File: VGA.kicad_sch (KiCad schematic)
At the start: 15 parts, among them U5 LMH6881SQ/NOPB

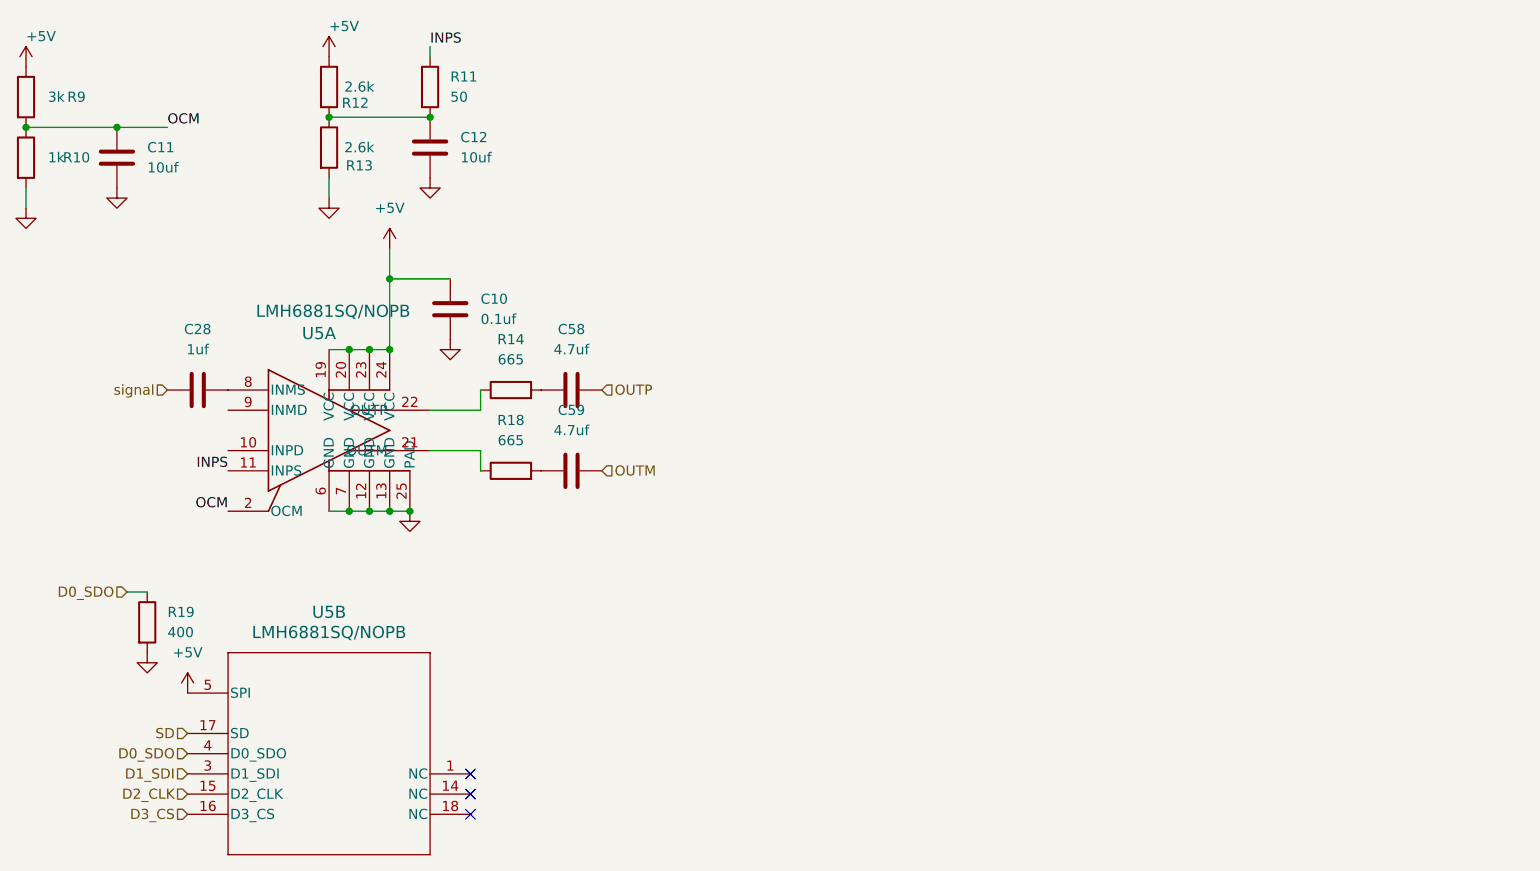
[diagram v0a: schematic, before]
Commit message: routing draft 2
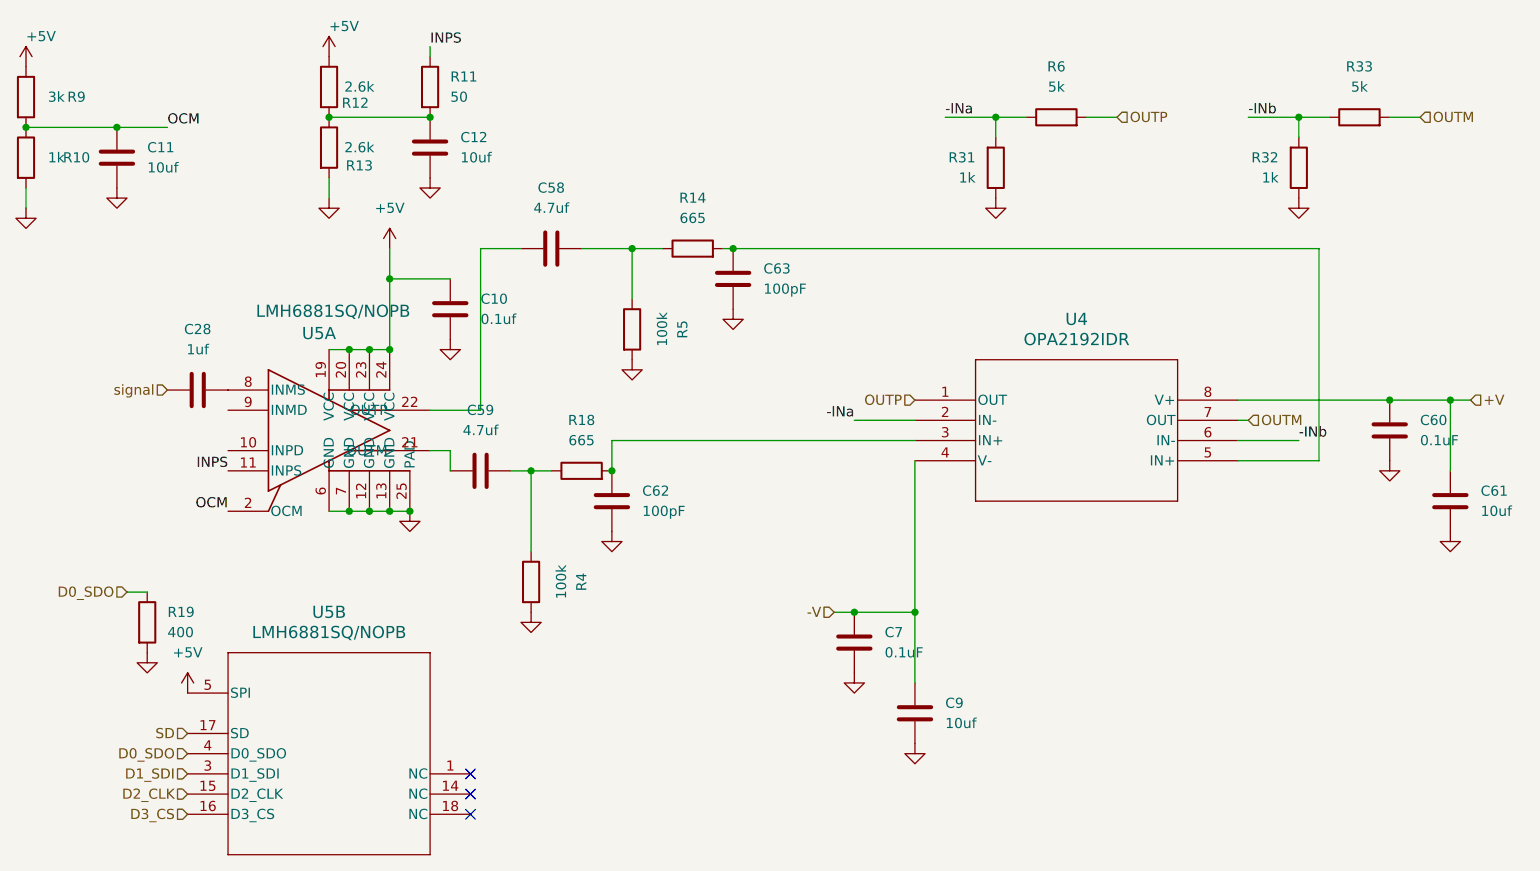
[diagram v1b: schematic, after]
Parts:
- added C60, C7: 0.1uF, Capacitor_SMD:C_0201_0603Metric, symbol Device:C
- added C61, C9: 10uf, Capacitor_THT:C_Radial_D5.0mm_H5.0mm_P2.00mm, symbol Device:C
- added C62, C63: 100pF, Capacitor_SMD:C_0805_2012Metric, symbol Device:C
- added R31, R32: 1k, Resistor_SMD:R_0805_2012Metric, symbol Device:R
- added R33, R6: 5k, Resistor_SMD:R_0805_2012Metric, symbol Device:R
- added R4, R5: 100k, Resistor_SMD:R_0805_2012Metric, symbol Device:R
- added U4: OPA2192IDR, DGK0008A_N_TEX, symbol 1_preamp:OPA2192IDR
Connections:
- net GND: now also C60.2, C61.2, C62.2, C63.2, C7.2, C9.2, R31.1, R32.1, R4.2, R5.2
- net OUTM: now also R33.2, U4.7 (OUT); no longer C59.1
- net OUTP: now also R6.2, U4.1 (OUT); no longer C58.1
- net at R14.2: now also C63.1, U4.5 (IN+); no longer C58.2
- net at R18.1: now also C59.1, R4.1; no longer U5.21 (OUTM)
- net at R18.2: now also C62.1, U4.3 (IN+); no longer C59.2
- net at R14.1: now also C58.1, R5.1; no longer U5.22 (OUTP)
- new net: C58.2, U5.22 (OUTP)
- new net: C59.2, U5.21 (OUTM)
- new net +V: C60.1, C61.1, U4.8 (V+)
- new net -INa: R31.2, R6.1, U4.2 (IN-)
- new net -INb: R32.2, R33.1, U4.6 (IN-)
- new net -V: C7.1, C9.1, U4.4 (V-)
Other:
- moved on the sheet: C58, C59, R14, R18
